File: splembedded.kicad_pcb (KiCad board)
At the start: 2 copper layers, 140 x 81.3 mm, 30 parts, among them SW1 Switch, SW10 Switch, SW11 Switch, SW12 Switch, SW13 Switch, SW14 Switch, SW15 Switch, SW2 Switch, SW3 Switch, SW4 Switch, SW5 Switch, SW6 Switch, SW7 Switch, SW8 Switch, SW9 Switch, U1 xiao-ble, U2 xiao-ble

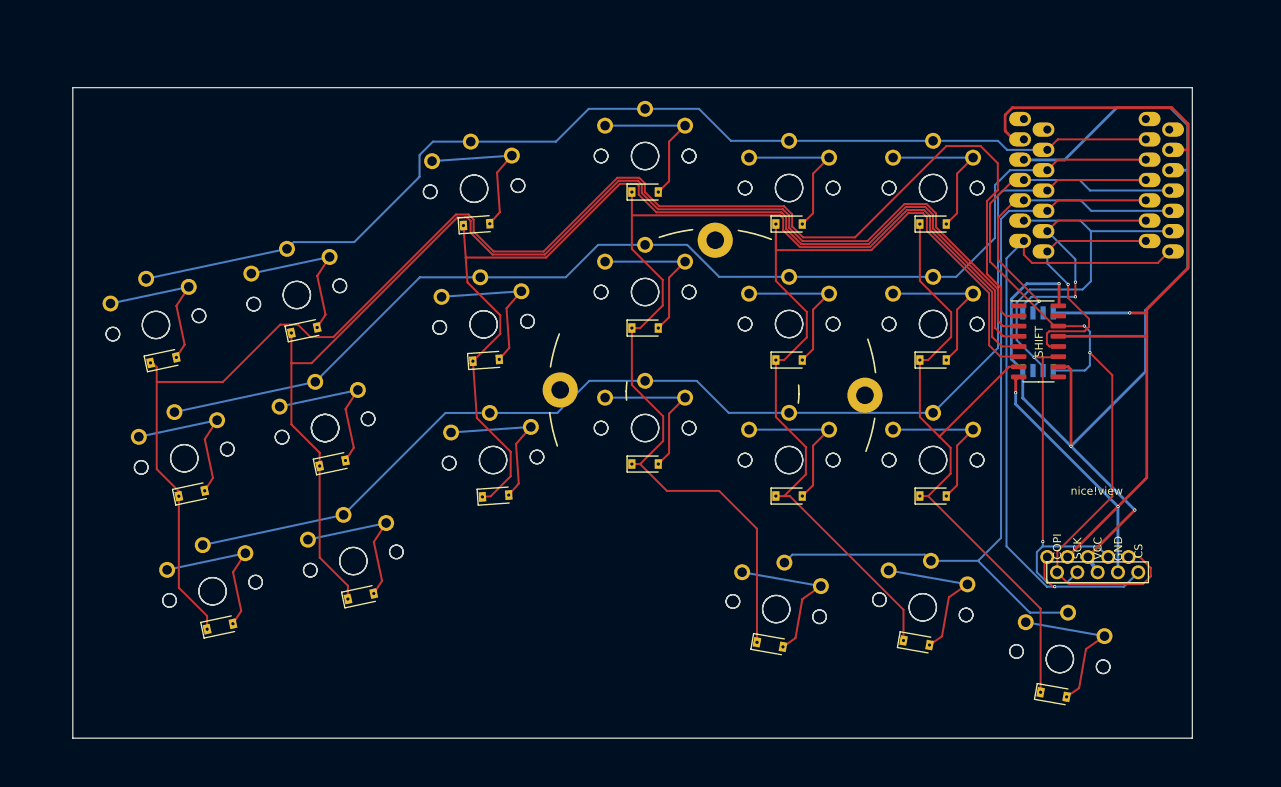
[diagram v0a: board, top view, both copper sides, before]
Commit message: smd branch init
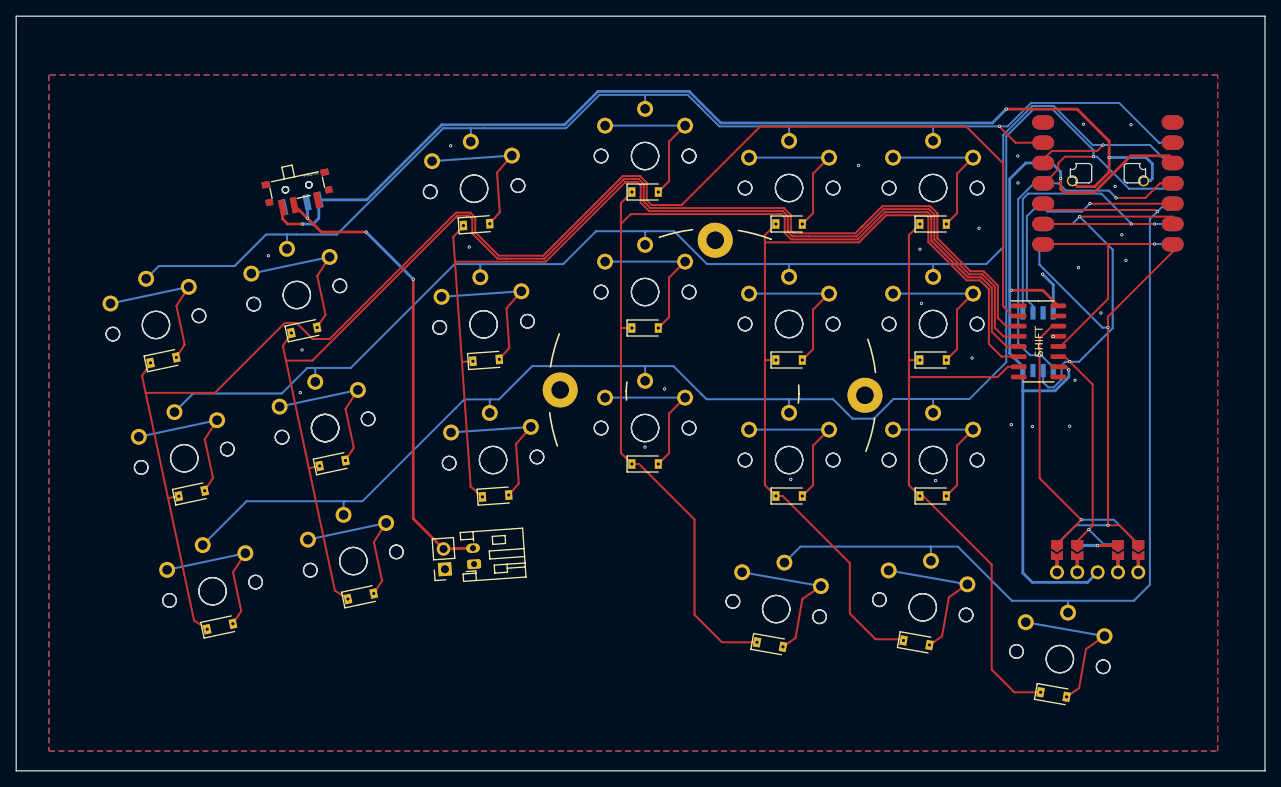
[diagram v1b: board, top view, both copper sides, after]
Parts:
- removed the display* at (186.3, 130.5)
- added J3: Pin Connector, Connector_PinSocket_2.54mm:PinSocket_1x02_P2.54mm_Vertical, F.Cu at (105.9, 148.5)
- added J4: JST Connector, Connector_JST:JST_PH_S2B-PH-K_1x02_P2.00mm_Horizontal, F.Cu at (109.6, 147.9)
- added RF*: JP, Jumper:SolderJumper-2_P1.3mm_Open_TrianglePad1.0x1.5mm, F.Cu at (182.4, 146.1)
- added RF*: JP, Jumper:SolderJumper-2_P1.3mm_Open_TrianglePad1.0x1.5mm, F.Cu at (192.6, 146.1)
- added RF*: JP, Jumper:SolderJumper-2_P1.3mm_Open_TrianglePad1.0x1.5mm, F.Cu at (185.0, 146.1)
- added RF*: JP, Jumper:SolderJumper-2_P1.3mm_Open_TrianglePad1.0x1.5mm, F.Cu at (190.1, 146.1)
- added RF*: JP, Jumper:SolderJumper-2_P1.3mm_Open_TrianglePad1.0x1.5mm, B.Cu at (190.1, 146.1)
- added RF*: JP, Jumper:SolderJumper-2_P1.3mm_Open_TrianglePad1.0x1.5mm, B.Cu at (192.6, 146.1)
- added RF*: JP, Jumper:SolderJumper-2_P1.3mm_Open_TrianglePad1.0x1.5mm, B.Cu at (185.0, 146.1)
- added RF*: JP, Jumper:SolderJumper-2_P1.3mm_Open_TrianglePad1.0x1.5mm, B.Cu at (182.4, 146.1)
- added SW2: SW_SPST, MSK-12C02:MSK-12C02, F.Cu at (87.5, 100.8)
- added SW2: SW_SPST, MSK-12C02:MSK-12C02, B.Cu at (87.5, 100.8)
- U1, U2: value xiao-ble -> xiao-ble-thruhole; footprint footprints:xiao-ble -> mcu:xiao-ble-smd-cutout
- moved U1 2.92 mm to (188.8, 100.3)
- moved U2 0.90 mm to (188.8, 100.3)
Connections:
- display* pad 1: COPI -> LCD_JP0
- display* pad 2: SCK -> LCD_JP1
- display* pad 4: GND -> LCD_JP2
- display* pad 5: LCD_CS -> LCD_JP3
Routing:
- net BAT+: track 0.00 -> 135.6 mm, vias 0 -> 3
- net GND: track 144.2 -> 10.6 mm, vias 3 -> 30
- net VBAT: track 0.00 -> 59.7 mm, vias 0 -> 3
- net R2: track 150.1 -> 188.4 mm, vias 0 -> 1
- net 3V3: track 136.8 -> 102.8 mm
- net R1: track 140.5 -> 172.9 mm, vias 0 -> 1
- net R0: track 136.9 -> 158.0 mm, vias 0 -> 1
- net COPI: track 105.2 -> 86.6 mm, vias 2 -> 3
- net LCD_CS: track 83.8 -> 66.3 mm, vias 1 -> 2
- net R3: track 101.9 -> 118.4 mm, vias 0 -> 1
- net FLASH_CS: track 30.5 -> 46.8 mm
- net SCK: track 90.4 -> 79.2 mm, vias 2 -> 3
- net CIPO: track 37.2 -> 32.6 mm
- net LCD_JP3: track 0.00 -> 4.12 mm
- net LCD_JP2: track 0.00 -> 4.12 mm
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- added copper zone on B.Cu, net GND
- added copper zone on F.Cu, net GND
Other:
- board size 140 x 81.3 mm -> 156.1 x 94.3 mm
